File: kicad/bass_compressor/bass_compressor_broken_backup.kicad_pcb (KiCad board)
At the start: 2 copper layers, 100 x 132 mm, 51 parts, among them IC1 NJM13700D, IC3 TC4013BP, J1 6.3mm TRS(mono use), J2 6.3mm TS(out), Q1 2SC1815, Q2 2SC1815, SW1 Cherry MX (手持ち), U1 TL072

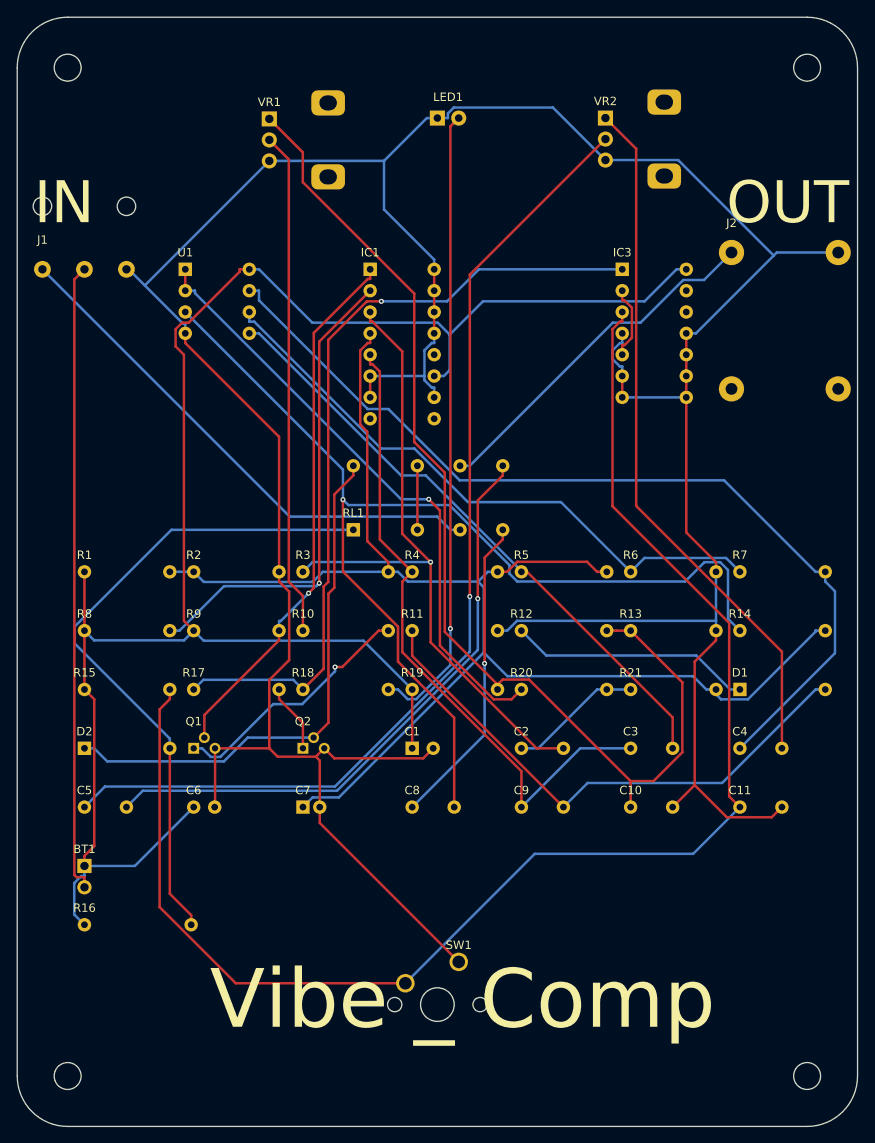
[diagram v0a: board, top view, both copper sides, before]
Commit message: PCB出力
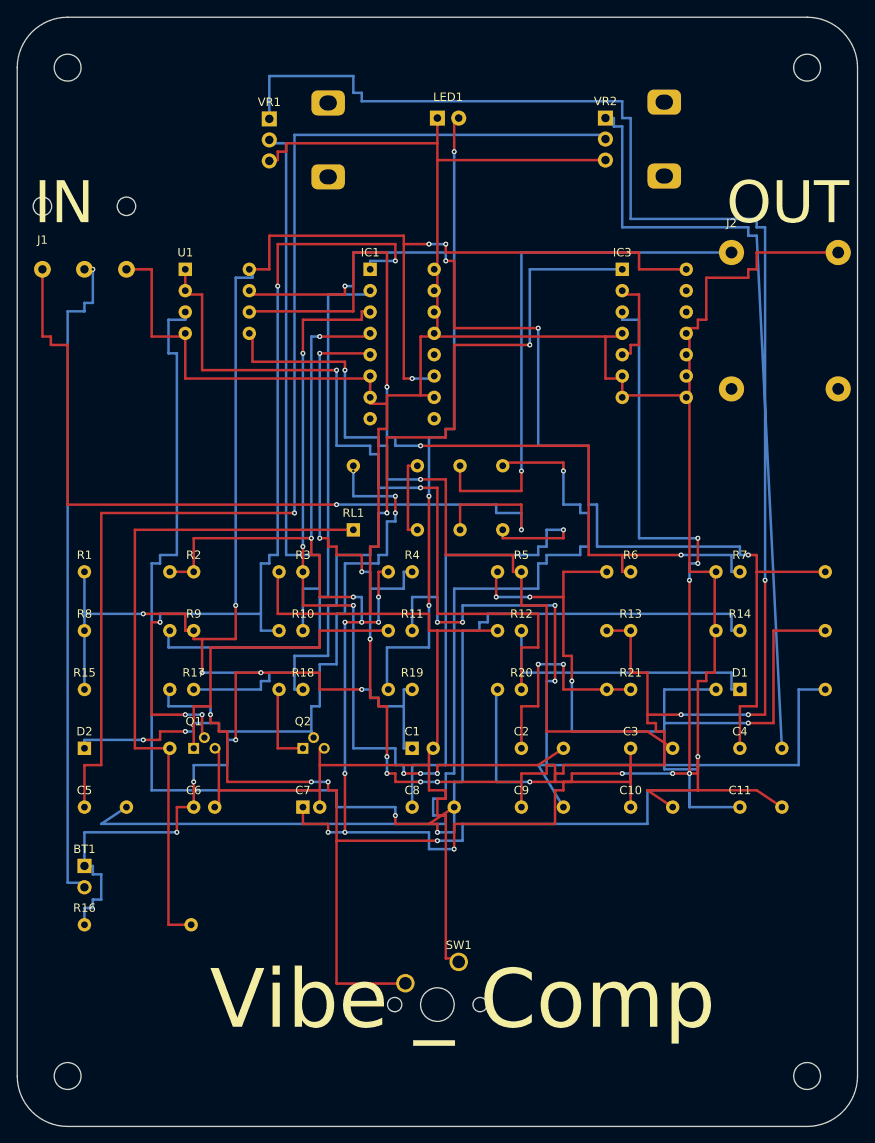
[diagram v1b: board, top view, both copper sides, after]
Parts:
- IC1: value NJM13700D -> LM13700
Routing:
- net VREF: track 170.2 -> 266.3 mm, vias 0 -> 18
- net ENV_B: track 130.8 -> 215.4 mm, vias 0 -> 4
- net WET_OUT: track 72.7 -> 118.2 mm
- net OTA_IABC1: track 64.2 -> 104.5 mm, vias 1 -> 5
- net IN_SIGNAL: track 62.5 -> 101.3 mm, vias 0 -> 2
- net BUF_IN: track 131.8 -> 169.7 mm, vias 1 -> 2
- net VPLUS: track 223.4 -> 258.2 mm, vias 0 -> 11
- net OTA_OUT: track 78.3 -> 112.2 mm, vias 0 -> 8
- net U1B_INN: track 73.2 -> 106.4 mm, vias 0 -> 3
- net GND: track 402.2 -> 432.9 mm
- net ENV_A: track 65.4 -> 96.0 mm, vias 0 -> 4
- net U1B_OUT: track 109.2 -> 134.8 mm, vias 0 -> 4
- net U1B_INP: track 73.0 -> 98.1 mm, vias 0 -> 2
- net WET_IN: track 37.5 -> 60.2 mm
- net BUF_OUT: track 72.8 -> 94.5 mm, vias 1 -> 2
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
